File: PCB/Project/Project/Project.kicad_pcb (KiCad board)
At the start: 2 copper layers, 10 parts, among them J1 Conn_01x03_Male, J2 DB9_Female, SW1 SW_Push, U1 ESP32-DEVKIT-V1

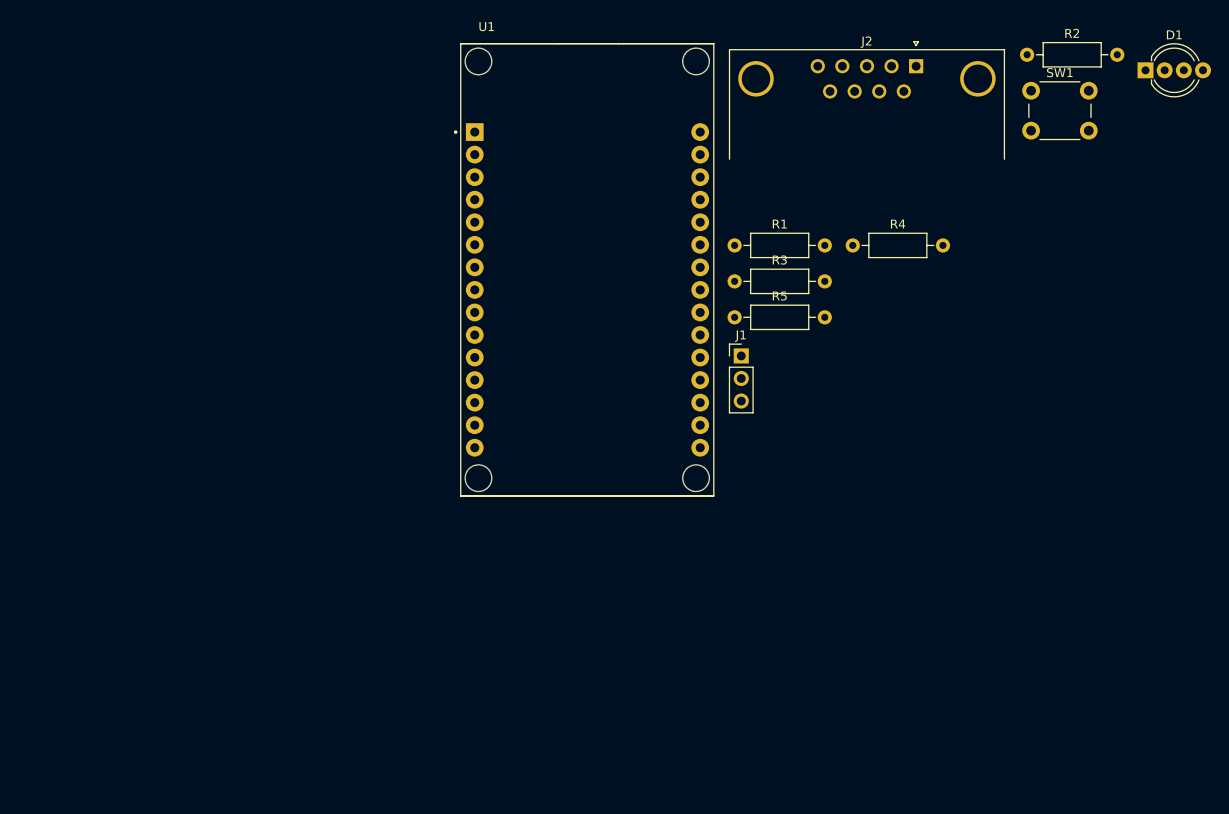
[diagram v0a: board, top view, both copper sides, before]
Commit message: Finished routing
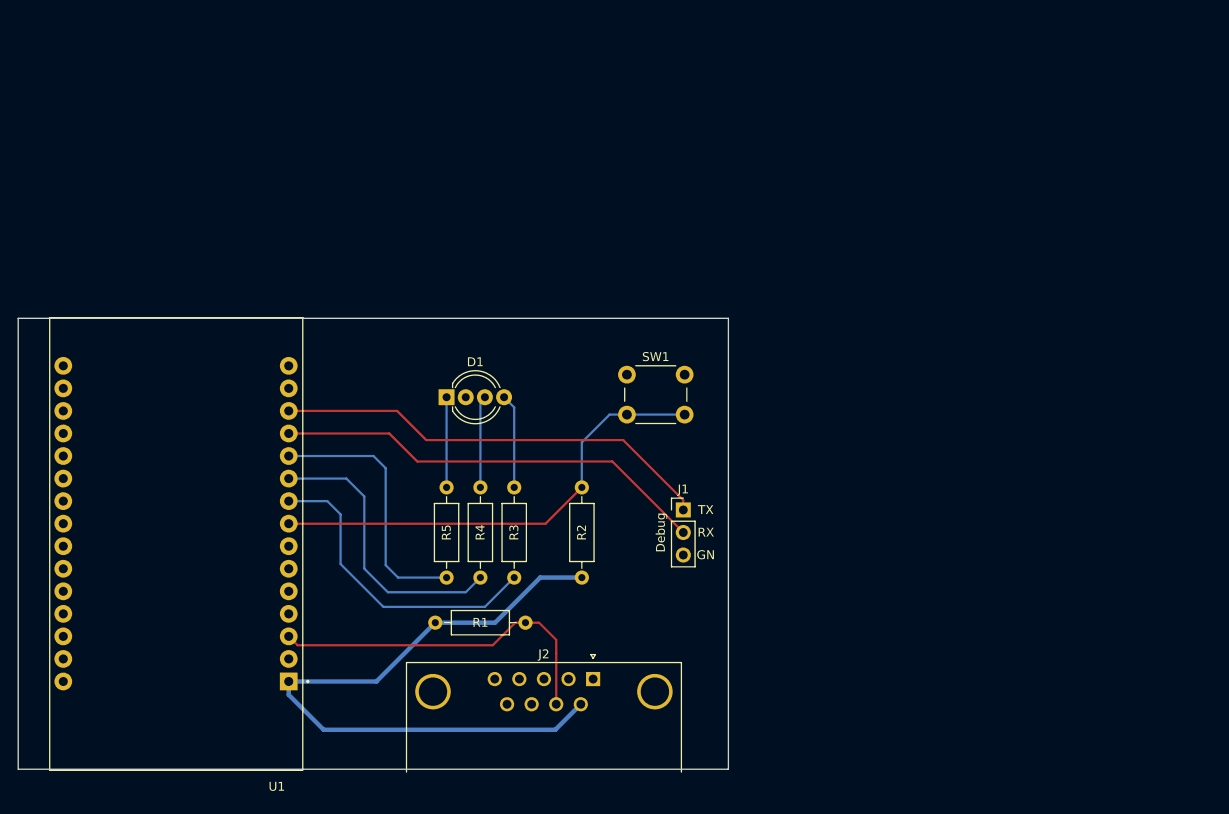
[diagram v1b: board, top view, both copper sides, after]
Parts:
- moved D1 86.9 mm to (85.1, 94.0)
- moved J2 78.0 mm to (101.6, 125.7)
- moved R2 77.4 mm to (100.3, 114.3), turned to 90 degrees
- moved U1 55.7 mm to (54.6, 110.5), turned to 180 degrees
- moved SW1 55.6 mm to (105.4, 91.4)
- moved R1 54.3 mm to (83.8, 119.4)
- moved R4 50.0 mm to (88.9, 104.1), turned to 270 degrees
- moved R5 37.7 mm to (85.1, 104.1), turned to 270 degrees
- moved R3 34.0 mm to (92.7, 104.1), turned to 270 degrees
- moved J1 18.5 mm to (111.8, 106.7)
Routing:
- net +3V3: track 0.00 -> 75.1 mm
- net BTN: track 0.00 -> 52.7 mm
- net TXD: track 0.00 -> 49.7 mm
- net RXD: track 0.00 -> 49.1 mm
- net DATA: track 0.00 -> 39.7 mm
- net LED_BLUE: track 0.00 -> 35.0 mm
- net LED_GREEN: track 0.00 -> 32.3 mm
- net LED_RED: track 0.00 -> 29.9 mm
- net Net-(D1-Pad4): track 0.00 -> 10.6 mm
- net Net-(D1-Pad3): track 0.00 -> 10.4 mm
- net Net-(D1-Pad1): track 0.00 -> 10.2 mm
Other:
- board outline added: 80 x 50.8 mm
- board text added: "Debug"
- board text added: "ESP32 Thermometer v0.1 Wojciech Zieliński 2022"
- board text added: "GN"
- board text added: "RX"
- board text added: "TX"
